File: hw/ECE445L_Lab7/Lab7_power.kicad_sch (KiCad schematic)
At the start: 9 parts, among them U3 RBT05W24S12

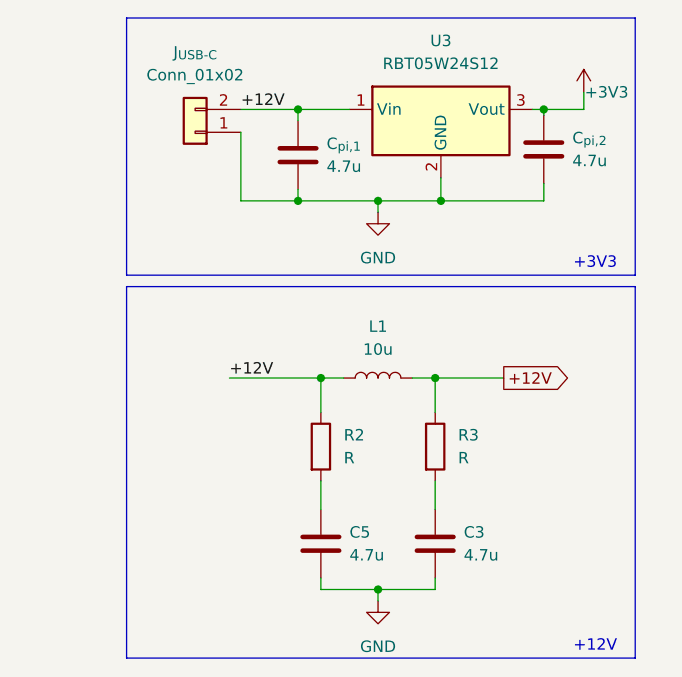
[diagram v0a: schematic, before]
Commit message: almost finished with schem
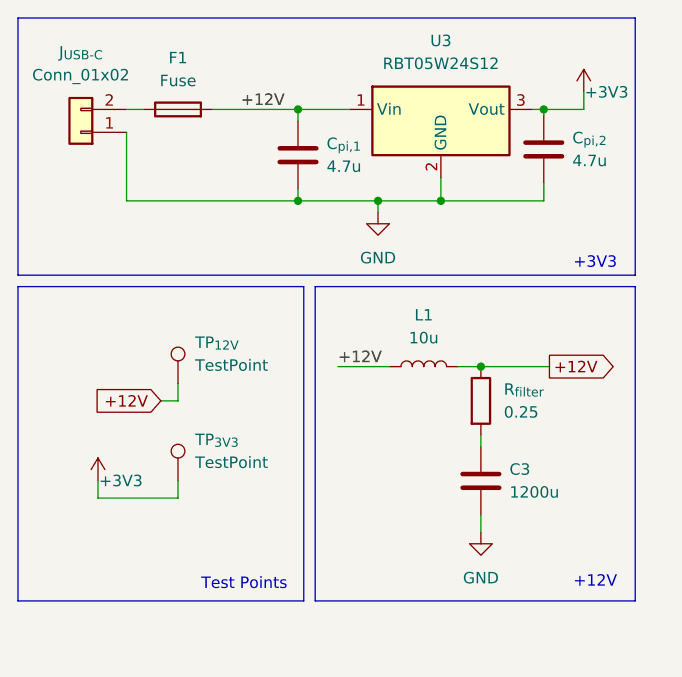
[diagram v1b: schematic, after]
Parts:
- removed C5: 4.7u, symbol Device:C
- removed R2: R, symbol Device:R
- added F1: Fuse, symbol Device:Fuse
- added TP_{12V}, TP_{3V3}: TestPoint, TestPoint:TestPoint_Bridge_Pitch2.0mm_Drill0.7mm, symbol Connector:TestPoint
- C3: value 4.7u -> 1200u
- L1: footprint (none) -> Inductor_SMD:L_APV_APH1040
- R_{filter}: renamed from R3; value R -> 0.25; footprint (none) -> Resistor_SMD:R_0603_1608Metric_Pad0.98x0.95mm_HandSolder
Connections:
- net +12V: now also F1.2, TP_{12V}.1; no longer J_{USB-C}.2 (Pin_2)
- net +3V3: now also TP_{3V3}.1
- new net: F1.1, J_{USB-C}.2 (Pin_2)
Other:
- note added: "Test Points"
- moved on the sheet: C3, J_{USB-C}, L1, R_{filter}
